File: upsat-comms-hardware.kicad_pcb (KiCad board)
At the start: 4 copper layers, 92.5 x 92.5 mm, 314 parts, among them U1 TXCO_TG_5021CG, U10 CC1120, U12 ADT7420, U14 OPA320, U16 RF5110G, U18 FA_128_, U2 TPS79930, U3 FA_128_, U4 CC1120, U5 STM32F407VG, U6 TXCO_TG_5021CG, U8 TPS79930, Y1 Crystal, Y2 Crystal

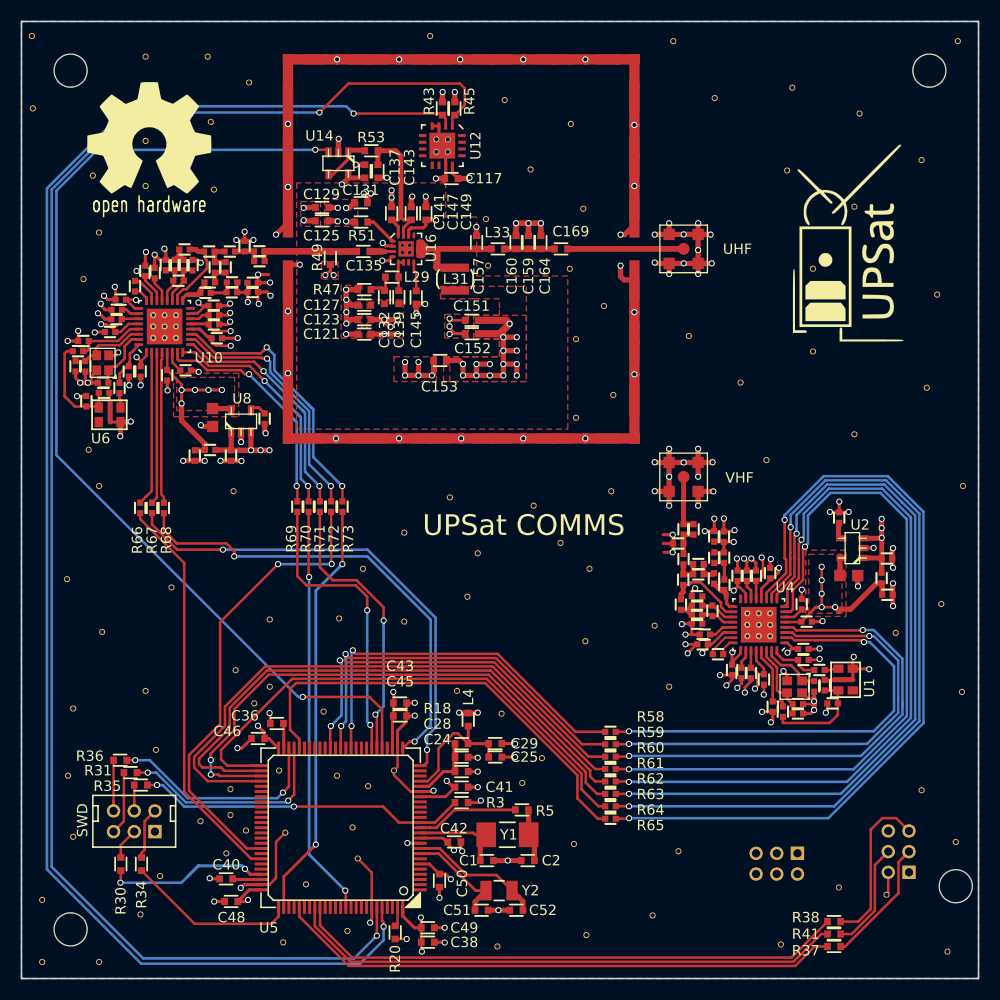
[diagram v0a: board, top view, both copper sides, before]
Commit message: Updating board
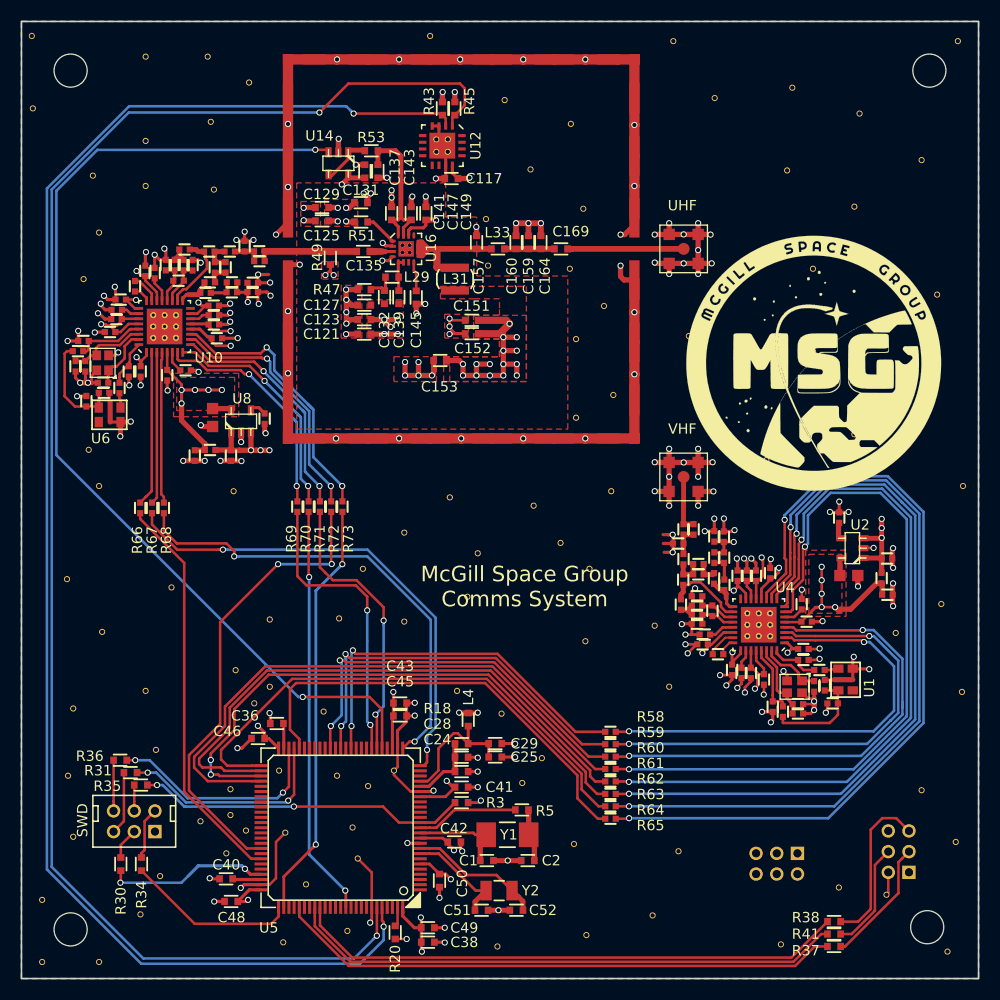
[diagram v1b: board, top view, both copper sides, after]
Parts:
- removed the G*** at (182.4, 76.0)
- removed the G*** at (114.8, 65.8)
- added G***: LOGO, libs:msg, F.Cu at (179.1, 87.6)
- moved REF** 4.83 mm to (190.0, 142.1)
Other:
- board text added: "McGill Space Group Comms System"
- board text added: "rip samosas 2019"
- board text removed: "In memory of K. Efstathiou"
- board text removed: "UPSat COMMS"
